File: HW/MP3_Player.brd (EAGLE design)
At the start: 210.9 x 16 mm, 79 parts, among them J2 LIPO-BATTERY-CONNECTOR, J3 USD-SDIO-SOCKETJLH, Q2 12.288MHz, U1 3.3V/150mA, U2 1.8V/100mA, U3 ATMEGA32U2, U4 VS1053B, U5 MCP73831

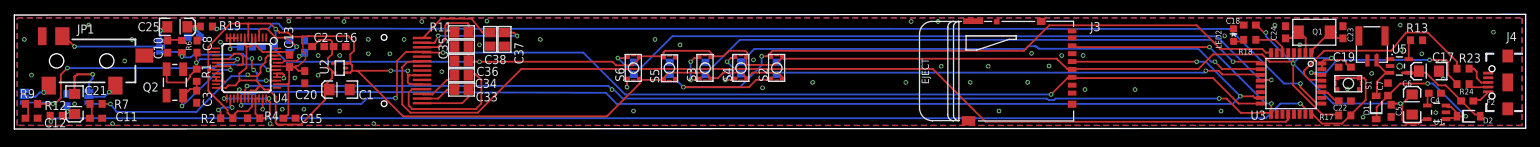
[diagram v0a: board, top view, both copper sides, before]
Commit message: gerber files generated
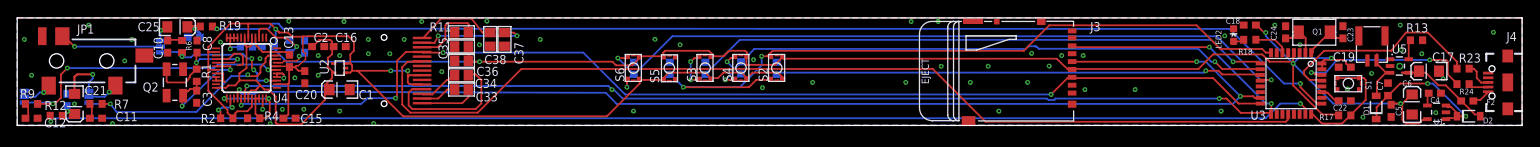
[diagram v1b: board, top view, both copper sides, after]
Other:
- board size 210.9 x 16 mm -> 210 x 15 mm
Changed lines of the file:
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@@
 <layer number="15" name="Route15" color="4" fill="6" visible="no" active="no"/>
 <layer number="16" name="Bottom" color="1" fill="1" visible="yes" active="yes"/>
-<layer number="17" name="Pads" color="2" fill="1" visible="yes" active="yes"/>
-<layer number="18" name="Vias" color="2" fill="1" visible="yes" active="yes"/>
-<layer number="19" name="Unrouted" color="6" fill="1" visible="yes" active="yes"/>
+<layer number="17" name="Pads" color="2" fill="1" visible="no" active="yes"/>
+<layer number="18" name="Vias" color="2" fill="1" visible="no" active="yes"/>
+<layer number="19" name="Unrouted" color="6" fill="1" visible="no" active="yes"/>
 <layer number="20" name="Dimension" color="15" fill="1" visible="yes" active="yes"/>
-<layer number="21" name="tPlace" color="7" fill="1" visible="yes" active="yes"/>
-<layer number="22" name="bPlace" color="7" fill="1" visible="yes" active="yes"/>
+<layer number="21" name="tPlace" color="7" fill="1" visible="no" active="yes"/>
+<layer number="22" name="bPlace" color="7" fill="1" visible="no" active="yes"/>
 <layer number="23" name="tOrigins" color="15" fill="1" visible="no" active="yes"/>
 <layer number="24" name="bOrigins" color="15" fill="1" visible="no" active="yes"/>
@@
 <description>Music player za ugradnju u hrbat knjige.</description>
 <plain>
-<wire x1="-0.4" y1="-0.5" x2="210.5" y2="-0.4" width="0" layer="20"/>
-<wire x1="210.5" y1="-0.4" x2="210.5" y2="15.5" width="0" layer="20"/>
-<wire x1="210.5" y1="15.5" x2="-0.4" y2="15.4" width="0" layer="20"/>
-<wire x1="-0.4" y1="15.4" x2="-0.4" y2="-0.5" width="0" layer="20"/>
+<wire x1="0" y1="0" x2="210" y2="0" width="0" layer="20"/>
+<wire x1="210" y1="0" x2="210" y2="15" width="0" layer="20"/>
+<wire x1="210" y1="15" x2="0" y2="15" width="0" layer="20"/>
+<wire x1="0" y1="15" x2="0" y2="0" width="0" layer="20"/>
 <wire x1="210" y1="0" x2="0" y2="0" width="0" layer="39"/>
-<dimension x1="0" y1="20" x2="210" y2="22" x3="105" y3="21" textsize="1.778" layer="20" dtype="horizontal" visible="yes"/>
-<dimension x1="86" y1="8" x2="91" y2="8" x3="88.5" y3="-9" textsize="1.27" layer="20" dtype="horizontal" extwidth="0.1" extlength="1" extoffset="8" precision="0" visible="yes"/>
-<dimension x1="91" y1="8" x2="96" y2="8" x3="93.5" y3="-9" textsize="1.27" layer="20" dtype="horizontal" extwidth="0.1" extlength="1" extoffset="8" precision="0" visible="yes"/>
-<dimension x1="96" y1="8" x2="101" y2="8" x3="98.5" y3="-9" textsize="1.27" layer="20" dtype="horizontal" extwidth="0.1" extlength="1" extoffset="8" precision="0" visible="yes"/>
-<dimension x1="101" y1="8" x2="106" y2="8" x3="103.5" y3="-9" textsize="1.27" layer="20" dtype="horizontal" extwidth="0.1" extlength="1" extoffset="8" precision="0" visible="yes"/>
-<dimension x1="50" y1="-10" x2="80" y2="-10" x3="65" y3="-7" textsize="1.27" layer="20" visible="yes"/>
-<dimension x1="0" y1="15" x2="0" y2="0" x3="-4" y3="7.5" textsize="1.27" layer="20" visible="yes"/>
-<dimension x1="0" y1="0" x2="50" y2="0" x3="25" y3="-7" textsize="1.27" layer="20" extoffset="3" visible="yes"/>
+<dimension x1="0" y1="20" x2="210" y2="22" x3="105" y3="21" textsize="1.778" layer="51" dtype="horizontal" visible="yes"/>
+<dimension x1="86" y1="8" x2="91" y2="8" x3="88.5" y3="-9" textsize="1.27" layer="51" dtype="horizontal" extwidth="0.1" extlength="1" extoffset="8" precision="0" visible="yes"/>
+<dimension x1="91" y1="8" x2="96" y2="8" x3="93.5" y3="-9" textsize="1.27" layer="51" dtype="horizontal" extwidth="0.1" extlength="1" extoffset="8" precision="0" visible="yes"/>
+<dimension x1="96" y1="8" x2="101" y2="8" x3="98.5" y3="-9" textsize="1.27" layer="51" dtype="horizontal" extwidth="0.1" extlength="1" extoffset="8" precision="0" visible="yes"/>
+<dimension x1="101" y1="8" x2="106" y2="8" x3="103.5" y3="-9" textsize="1.27" layer="51" dtype="horizontal" extwidth="0.1" extlength="1" extoffset="8" precision="0" visible="yes"/>
+<dimension x1="50" y1="-10" x2="80" y2="-10" x3="65" y3="-7" textsize="1.27" layer="51" visible="yes"/>
+<dimension x1="0" y1="15" x2="0" y2="0" x3="-4" y3="7.5" textsize="1.27" layer="51" visible="yes"/>
+<dimension x1="0" y1="0" x2="50" y2="0" x3="25" y3="-7" textsize="1.27" layer="51" extoffset="3" visible="yes"/>
 </plain>
 <attributes>
